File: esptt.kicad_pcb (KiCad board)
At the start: 2 copper layers, 21.3 x 43 mm, 17 parts

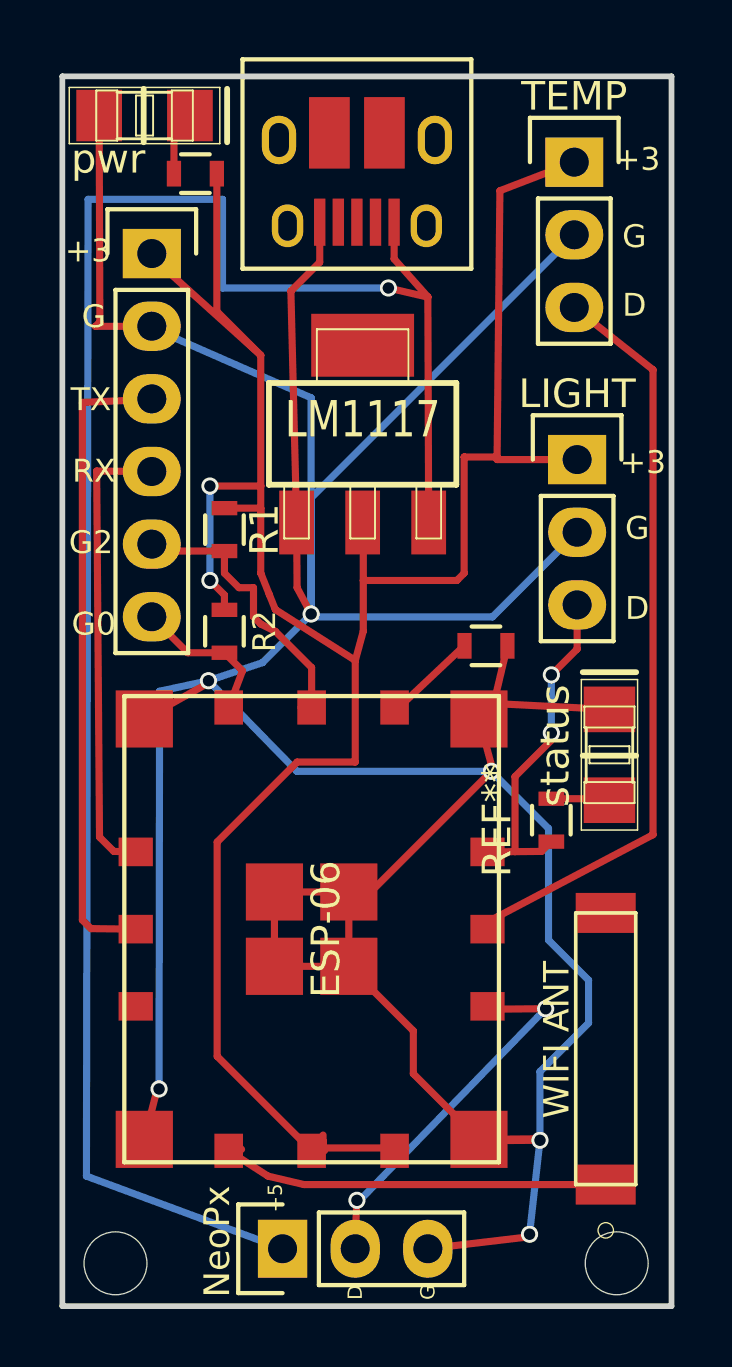
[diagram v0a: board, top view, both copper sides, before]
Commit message: tweaks
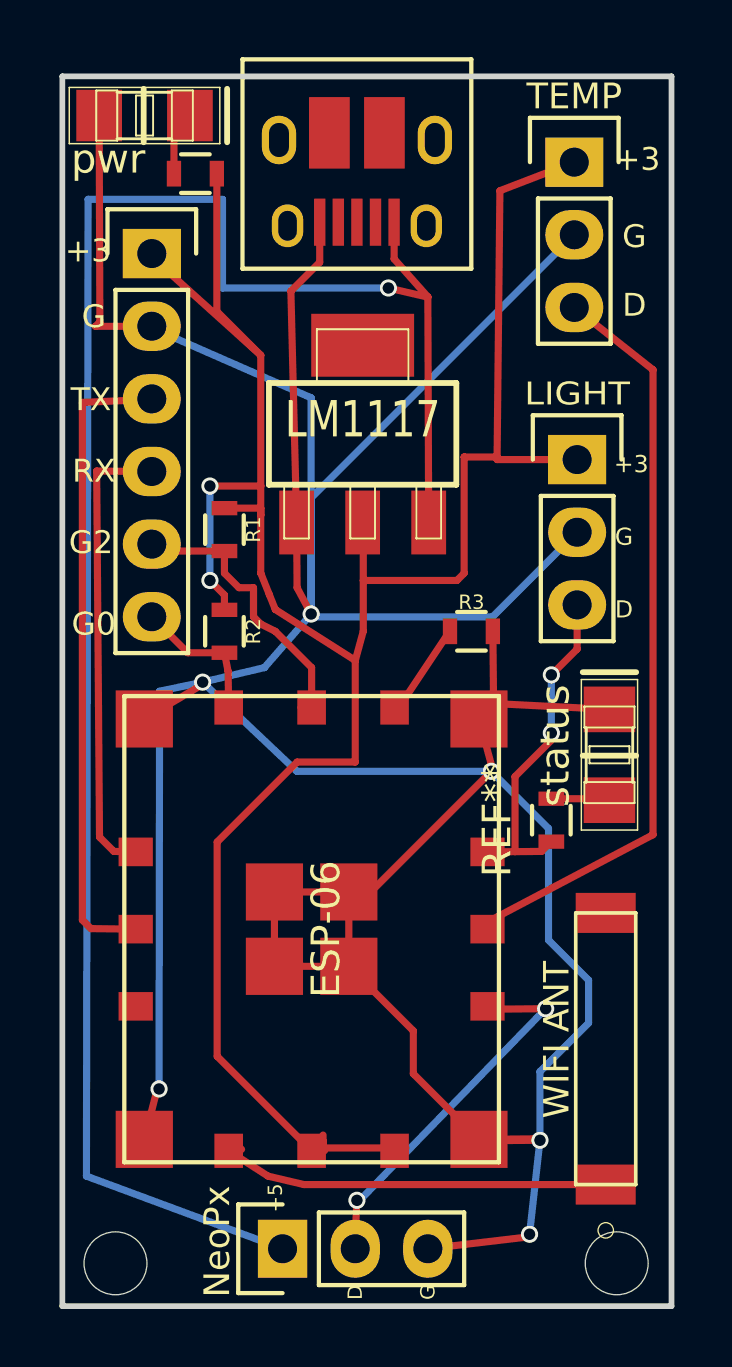
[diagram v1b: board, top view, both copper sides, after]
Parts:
- moved R3 0.72 mm to (146.3, 57.4)
- gave numbers to parts that had none: 1
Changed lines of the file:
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@@
     (34 B.Paste user hide)
     (35 F.Paste user)
-    (36 B.SilkS user hide)
+    (36 B.SilkS user)
     (37 F.SilkS user)
     (38 B.Mask user)
@@
     (tags "resistor 0603")
     (attr smd)
-    (fp_text reference R2 (at 0 1.4 90) (layer F.SilkS)
-      (effects (font (size 0.8 0.8) (thickness 0.1)))
+    (fp_text reference R2 (at 0 1.016 90) (layer F.SilkS)
+      (effects (font (size 0.5 0.5) (thickness 0.1)))
     )
     (fp_text value R_0603 (at 0 1.9 90) (layer F.Fab)
@@
     (tags "pin header")
     (fp_text reference TEMP (at 0 -2.3) (layer F.SilkS)
-      (effects (font (size 1 1) (thickness 0.15)))
+      (effects (font (size 0.9 0.9) (thickness 0.1)))
     )
     (fp_text value Pin_Header_Straight_1x03 (at 0 -3.1) (layer F.Fab) hide
@@
     (tags "pin header")
     (fp_text reference LIGHT (at 0 -2.3) (layer F.SilkS)
-      (effects (font (size 1 1) (thickness 0.15)))
+      (effects (font (size 0.8 0.9) (thickness 0.15)))
     )
     (fp_text value Pin_Header_Straight_1x03 (at 0 -3.1) (layer F.Fab) hide
@@
     (tags "resistor 0603")
     (attr smd)
-    (fp_text reference R1 (at 0 1.4 90) (layer F.SilkS)
-      (effects (font (size 1 1) (thickness 0.15)))
+    (fp_text reference R1 (at 0 1.016 90) (layer F.SilkS)
+      (effects (font (size 0.5 0.5) (thickness 0.1)))
     )
     (fp_text value R_0603 (at 0 1.9 90) (layer F.Fab)
@@
   )
   (module Resistors_SMD:R_0603 (layer F.Cu)
-    (at 146.812 57.912)
+    (at 146.304 57.404)
     (descr "Resistor SMD 0603, reflow soldering, Vishay (see dcrcw.pdf)")
     (tags "resistor 0603")
     (attr smd)
-    (fp_text reference "" (at 0 -1.9) (layer F.SilkS)
-      (effects (font (size 1 1) (thickness 0.15)))
+    (fp_text reference R3 (at 0 -1.016) (layer F.SilkS)
+      (effects (font (size 0.5 0.5) (thickness 0.1)))
     )
     (fp_text value R_0603 (at 0 1.9) (layer F.Fab)
@@
       (rotate (xyz 0 0 0))
     )
+    (model Resistors_SMD.3dshapes/R_0603.wrl
+      (at (xyz 0 0 0))
+      (scale (xyz 1 1 1))
+      (rotate (xyz 0 0 0))
+    )
   )
   (module Resistors_SMD:R_0603 (layer F.Cu)
@@
     (effects (font (size 0.8 0.8) (thickness 0.2)))
   )
-  (gr_text D (at 152.1 56.6) (layer F.SilkS)
-    (effects (font (size 0.8 0.8) (thickness 0.2)))
+  (gr_text D (at 151.638 56.642) (layer F.SilkS)
+    (effects (font (size 0.6 0.6) (thickness 0.1)))
   )
   (gr_text D (at 152 46) (layer F.SilkS)
     (effects (font (size 0.8 0.8) (thickness 0.2)))
   )
-  (gr_text G (at 152.1 53.8) (layer F.SilkS)
-    (effects (font (size 0.8 0.8) (thickness 0.2)))
+  (gr_text G (at 151.638 54.102) (layer F.SilkS)
+    (effects (font (size 0.6 0.6) (thickness 0.1)))
   )
   (gr_text G (at 152 43.6) (layer F.SilkS)
@@
     (effects (font (size 0.5 0.5) (thickness 0.125)))
   )
-  (gr_text +3 (at 152.3 51.5) (layer F.SilkS)
-    (effects (font (size 0.8 0.8) (thickness 0.2)))
+  (gr_text +3 (at 151.892 51.562) (layer F.SilkS)
+    (effects (font (size 0.6 0.6) (thickness 0.1)))
   )
   (gr_text +3 (at 152.1 40.9) (layer F.SilkS)
@@
   (via (at 137.16 55.626) (size 0.6) (drill 0.4) (layers F.Cu B.Cu) (net 0))
   (segment (start 137.668 56.134) (end 137.16 55.626) (width 0.25) (layer F.Cu) (net 0))
-  (segment (start 137.816 60.068) (end 138.3 58.786) (width 0.25) (layer F.Cu) (net 0) (status 10))
-  (segment (start 138.3 58.786) (end 137.668 58.154) (width 0.25) (layer F.Cu) (net 0) (status 20))
+  (segment (start 137.816 60.068) (end 137.795 58.801) (width 0.25) (layer F.Cu) (net 0) (status 400010))
+  (segment (start 137.795 58.801) (end 137.668 58.154) (width 0.25) (layer F.Cu) (net 0) (status 800020))
   (segment (start 135.37 56.654) (end 135.128 56.896) (width 0.25) (layer F.Cu) (net 0) (status 30))
   (segment (start 137.668 54.598) (end 135.37 54.598) (width 0.25) (layer F.Cu) (net 0) (status 30))
@@
   (segment (start 137.668 53.098) (end 138.938 53.098) (width 0.25) (layer F.Cu) (net 0) (status 10))
   (segment (start 138.938 53.098) (end 138.938 53.34) (width 0.25) (layer F.Cu) (net 0))
-  (segment (start 147.562 57.912) (end 147.078 59.956) (width 0.25) (layer F.Cu) (net 0) (status 30))
+  (segment (start 147.054 57.404) (end 147.078 59.956) (width 0.25) (layer F.Cu) (net 0) (status 30))
   (segment (start 147.078 59.956) (end 146.566 60.468) (width 0.25) (layer F.Cu) (net 0) (status 30))
   (segment (start 135.14 54.368) (end 135.128 54.356) (width 0.25) (layer F.Cu) (net 0) (status 30))
@@
   (segment (start 147.1035 59.9305) (end 146.566 60.468) (width 0.25) (layer F.Cu) (net 0) (status 30))
   (segment (start 143.616 60.068) (end 143.766 60.068) (width 0.25) (layer F.Cu) (net 0) (status 30))
-  (segment (start 143.766 60.068) (end 146.05 57.912) (width 0.25) (layer F.Cu) (net 0) (status 30))
+  (segment (start 143.766 60.068) (end 145.542 57.404) (width 0.25) (layer F.Cu) (net 0) (status 30))
   (segment (start 144.78 45.72) (end 143.4 45.4) (width 0.25) (layer F.Cu) (net 0))
   (segment (start 132.842 76.454) (end 139.7 78.994) (width 0.25) (layer B.Cu) (net 0) (status 20))
@@
   (segment (start 142.4 77.3) (end 148.9 70.6) (width 0.25) (layer B.Cu) (net 0))
   (segment (start 147 62.3) (end 140.2 62.3) (width 0.25) (layer B.Cu) (net 0))
-  (segment (start 140.2 62.3) (end 137.11 59.132) (width 0.25) (layer B.Cu) (net 0))
+  (segment (start 140.2 62.3) (end 136.906 59.182) (width 0.25) (layer B.Cu) (net 0))
   (segment (start 147.05 62.25) (end 146.566 60.468) (width 0.25) (layer F.Cu) (net 0) (status 20))
   (via (at 147 62.3) (size 0.6) (drill 0.4) (layers F.Cu B.Cu) (net 0))
@@
   (segment (start 135.382 73.406) (end 135.4 59.5) (width 0.25) (layer B.Cu) (net 0))
   (via (at 135.382 73.406) (size 0.6) (drill 0.4) (layers F.Cu B.Cu) (net 0))
-  (segment (start 134.866 75.168) (end 135.332 73.356) (width 0.25) (layer F.Cu) (net 0) (status 400010))
+  (segment (start 134.866 75.168) (end 135.332 73.356) (width 0.25) (layer F.Cu) (net 0) (status 10))
   (segment (start 135.332 73.356) (end 135.382 73.406) (width 0.25) (layer F.Cu) (net 0))
-  (segment (start 135.4 59.5) (end 137.11 59.132) (width 0.25) (layer B.Cu) (net 0))
+  (segment (start 135.4 59.5) (end 136.906 59.182) (width 0.25) (layer B.Cu) (net 0))
   (segment (start 142.24 78.634) (end 142.24 78.994) (width 0.25) (layer B.Cu) (net 0) (status 30))
   (segment (start 137.816 75.568) (end 139.192 76.454) (width 0.25) (layer F.Cu) (net 0) (status 10))
@@
   (segment (start 140.7 56.8) (end 140.7 49.24) (width 0.25) (layer B.Cu) (net 0))
   (segment (start 140.7 49.24) (end 135 46.74) (width 0.25) (layer B.Cu) (net 0) (status 20))
-  (segment (start 137.11 59.132) (end 139 58.5) (width 0.25) (layer B.Cu) (net 0))
-  (segment (start 139 58.5) (end 140.7 56.8) (width 0.25) (layer B.Cu) (net 0))
-  (segment (start 137.16 59.182) (end 137.11 59.132) (width 0.25) (layer F.Cu) (net 0))
-  (via (at 137.11 59.132) (size 0.6) (drill 0.4) (layers F.Cu B.Cu) (net 0))
-  (segment (start 134.866 60.468) (end 137.16 59.182) (width 0.25) (layer F.Cu) (net 0) (status 10))
+  (segment (start 136.906 59.182) (end 139.065 58.674) (width 0.25) (layer B.Cu) (net 0))
+  (segment (start 139.065 58.674) (end 140.7 56.8) (width 0.25) (layer B.Cu) (net 0))
+  (segment (start 136.956 59.232) (end 136.906 59.182) (width 0.25) (layer F.Cu) (net 0))
+  (via (at 136.906 59.182) (size 0.6) (drill 0.4) (layers F.Cu B.Cu) (net 0))
+  (segment (start 134.866 60.468) (end 136.956 59.232) (width 0.25) (layer F.Cu) (net 0) (status 400010))
   (segment (start 140.208 55.88) (end 140.7 56.8) (width 0.25) (layer F.Cu) (net 0))
   (via (at 140.7 56.8) (size 0.6) (drill 0.4) (layers F.Cu B.Cu) (net 0))
